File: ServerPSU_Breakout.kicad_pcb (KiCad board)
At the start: 2 copper layers, 91.4 x 69.8 mm, 4 parts

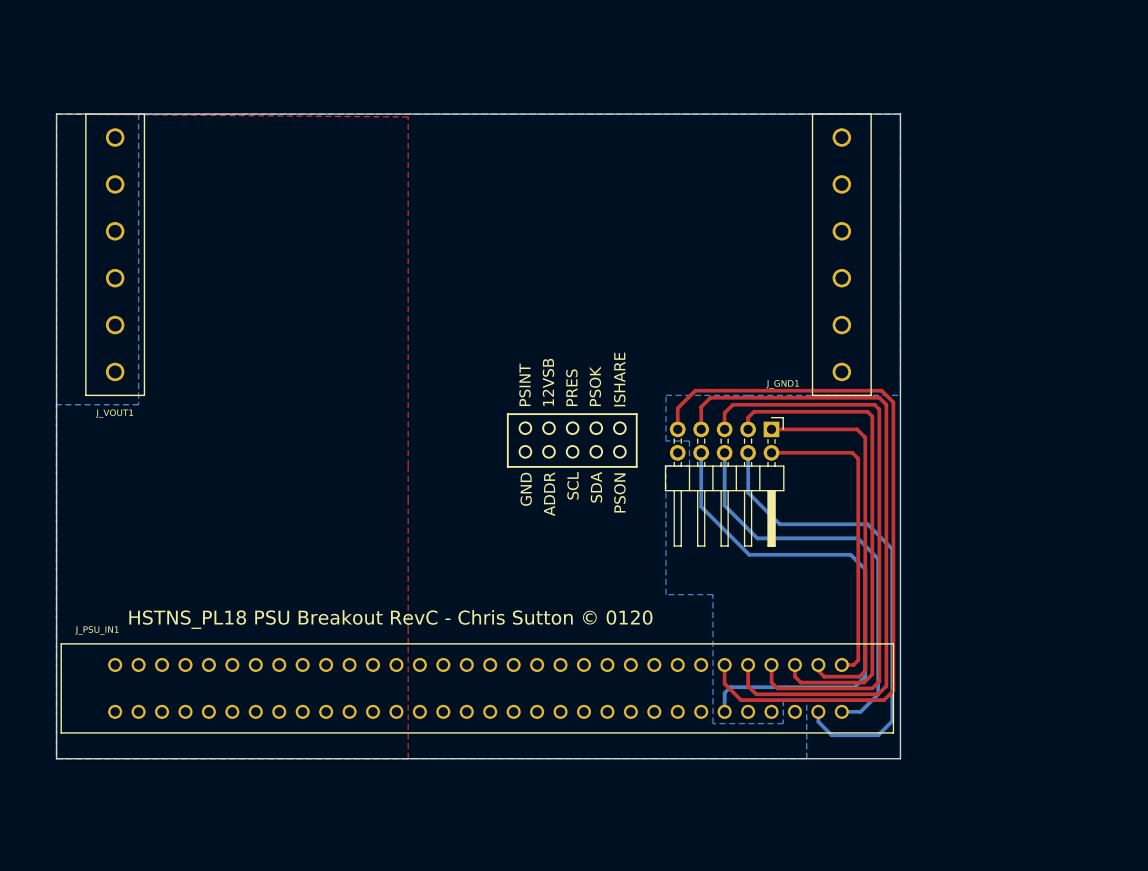
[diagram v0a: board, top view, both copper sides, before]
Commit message: layout draft
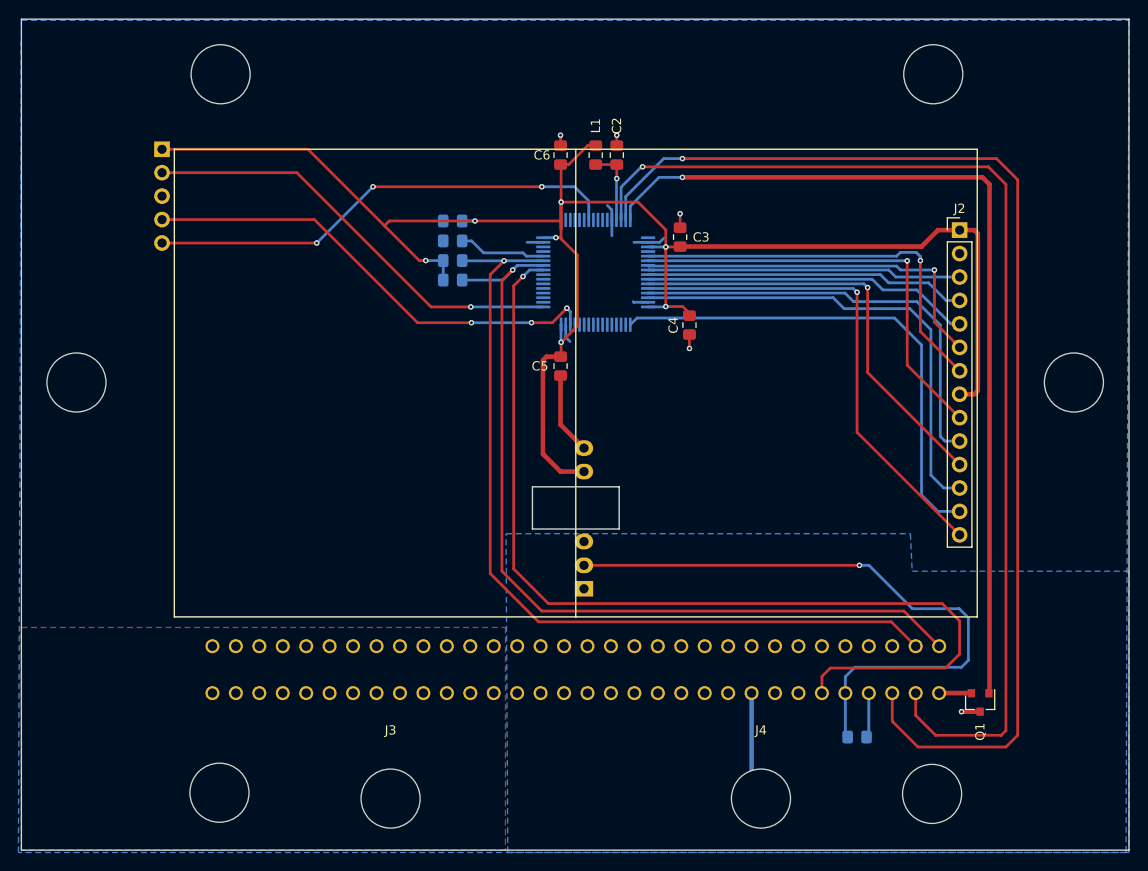
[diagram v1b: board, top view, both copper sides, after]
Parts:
- removed J_DATA1: 2x5_2.54mm, Connector_PinHeader_2.54mm:PinHeader_2x05_P2.54mm_Horizontal
- removed J_GND1, J_VOUT1: 1x6_5.08mm, Samtec HPM-06-02-T-S-RA_1x6:Samtec HPM-06-02-T-S-RA_2x6
- added C1: 100nF, Capacitor_SMD:C_0805_2012Metric_Pad1.15x1.40mm_HandSolder, B.Cu at (148.3, 68.7)
- added C2: 100nF, Capacitor_SMD:C_0805_2012Metric_Pad1.15x1.40mm_HandSolder, F.Cu at (166.1, 61.6)
- added C3: 100nF, Capacitor_SMD:C_0805_2012Metric_Pad1.15x1.40mm_HandSolder, F.Cu at (173.0, 70.5)
- added C4: 100nF, Capacitor_SMD:C_0805_2012Metric_Pad1.15x1.40mm_HandSolder, F.Cu at (174.0, 80.0)
- added C5: 100nF, Capacitor_SMD:C_0805_2012Metric_Pad1.15x1.40mm_HandSolder, F.Cu at (160.0, 84.5)
- added C6: 100nF, Capacitor_SMD:C_0805_2012Metric_Pad1.15x1.40mm_HandSolder, F.Cu at (160.0, 61.6)
- added J1: Conn_01x05, Connector_PinHeader_2.54mm:PinHeader_1x05_P2.54mm_Vertical, B.Cu at (116.8, 61.0)
- added J2: Conn_01x14, Connector_PinHeader_2.54mm:PinHeader_1x14_P2.54mm_Vertical, F.Cu at (203.3, 69.7)
- added J3: Conn_01x01, MountingHole:MountingHole_6.4mm_M6, F.Cu at (141.6, 131.3)
- added J4: Conn_01x01, MountingHole:MountingHole_6.4mm_M6, F.Cu at (181.7, 131.3)
- added L1: BEAD, Inductor_SMD:L_0805_2012Metric_Pad1.15x1.40mm_HandSolder, F.Cu at (163.8, 61.6)
- added Q1: DMG2302U, Package_TO_SOT_SMD:SOT-23, F.Cu at (205.5, 120.9)
- added R1: 10K, Resistor_SMD:R_0805_2012Metric_Pad1.15x1.40mm_HandSolder, B.Cu at (148.3, 75.1)
- added R2: 10K, Resistor_SMD:R_0805_2012Metric_Pad1.15x1.40mm_HandSolder, B.Cu at (148.3, 73.0)
- added R3: 22K, Resistor_SMD:R_0805_2012Metric_Pad1.15x1.40mm_HandSolder, B.Cu at (192.2, 124.7)
- added R4: 10K, Resistor_SMD:R_0805_2012Metric_Pad1.15x1.40mm_HandSolder, B.Cu at (148.3, 70.9)
- added REF**: MountingHole_6.4mm_M6, MountingHole:MountingHole_6.4mm_M6, F.Cu at (215.6, 86.2)
- added REF**: MountingHole_6.4mm_M6, MountingHole:MountingHole_6.4mm_M6, F.Cu at (107.6, 86.2)
- added REF**: MountingHole_6.4mm_M6, MountingHole:MountingHole_6.4mm_M6, F.Cu at (200.3, 130.8)
- added REF**: MountingHole_6.4mm_M6, MountingHole:MountingHole_6.4mm_M6, F.Cu at (123.1, 130.7)
- added REF**: MountingHole_6.4mm_M6, MountingHole:MountingHole_6.4mm_M6, F.Cu at (200.4, 52.8)
- added REF**: MountingHole_6.4mm_M6, MountingHole:MountingHole_6.4mm_M6, F.Cu at (123.2, 52.8)
- added U1: NCS1S1203SC, Converter_DCDC:Converter_DCDC_Murata_NCS1SxxxxSC_THT, B.Cu at (162.6, 108.6)
- added U2: STM32F072RBTx, Package_QFP:LQFP-64_10x10mm_P0.5mm, B.Cu at (163.8, 74.3)
- J_PSU_IN1: moved to B.Cu
- moved J_PSU_IN1 10.7 mm to (161.7, 117.3), turned to 270 degrees
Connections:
- net /12V renamed /OutputConnectors/PSU_VBUS
- net /GND renamed GNDS
- J_PSU_IN1 pad 27: /ADDR -> /PSUConnector/PSU_ADDR2
- J_PSU_IN1 pad 28: Net-(J_PSU_IN1-Pad28) -> /PSUConnector/PSU_ADDR1
- J_PSU_IN1 pad 29: Net-(J_PSU_IN1-Pad29) -> /PSUConnector/PSU_ADDR0
- J_PSU_IN1 pad 31: /SDA -> /PSUConnector/PSU_SDA
- J_PSU_IN1 pad 32: /SCL -> /PSUConnector/PSU_SCL
- J_PSU_IN1 pad 33: /PSON -> /HighVoltageControl/PSU_ON
- J_PSU_IN1 pad 34: /ISHARE -> /MCU/MCU_IMON
- J_PSU_IN1 pad 35: /PSOK -> /MCU/MCU_PSOK
- J_PSU_IN1 pad 36: /PRESENT -> /HighVoltageControl/PSU_PRES
- J_PSU_IN1 pad 37: /12VSB -> /HighVoltageControl/PSU_12VSB
- J_PSU_IN1 pad 38: /PSINTERRUPT -> /PSUConnector/PSU_INT
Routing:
- net /HighVoltageControl/MCU_3V3: track 0.00 -> 193.4 mm, vias 0 -> 7
- net /MCU/MCU_PSOK: track 0.00 -> 126.2 mm, vias 0 -> 1
- net /MCU/MCU_IMON: track 0.00 -> 119.4 mm, vias 0 -> 1
- net /PSUConnector/PSU_INT: track 0.00 -> 106.6 mm, vias 0 -> 1
- net /HighVoltageControl/MCU_SW: track 0.00 -> 97.2 mm, vias 0 -> 1
- net /PSUConnector/PSU_SCL: track 0.00 -> 93.3 mm, vias 0 -> 1
- net /PSUConnector/PSU_SDA: track 0.00 -> 92.7 mm, vias 0 -> 1
- net /PSINTERRUPT: track 79.7 -> 0.00 mm
- net /12VSB: track 71.7 -> 0.00 mm
- net /HighVoltageControl/PSU_12VSB: track 0.00 -> 69.4 mm, vias 0 -> 1
- net /PRESENT: track 62.8 -> 0.00 mm
- net /ADDR: track 56.1 -> 0.00 mm
- net /MCU/T_OUT: track 0.00 -> 54.2 mm
- net /MCU/T_IRQ: track 0.00 -> 53.7 mm, vias 0 -> 1
- net /PSOK: track 53.4 -> 0.00 mm
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- added copper zone on B.Cu, net /HighVoltageControl/MCU_GND
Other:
- board size 91.4 x 69.8 mm -> 120 x 90 mm
- net class Default: clearance 0.2 -> 0.127; trace_width 0.25 -> 0.127; via_dia 0.8 -> 0.6; via_drill 0.4 -> 0.3
- rule trace_clearance: 0.2 -> 0.127
- rule trace_min: 0.2 -> 0.127
- rule via_min_size: 0.4 -> 0.6
- board text removed: "12VSB"
- board text removed: "ADDR"
- board text removed: "GND"
- board text removed: "HSTNS_PL18 PSU Breakout RevC - Chris Sutton © 0120"
- board text removed: "ISHARE"
- board text removed: "PRES"
- board text removed: "PSINT"
- board text removed: "PSOK"
- board text removed: "PSON"
- board text removed: "SCL"
- board text removed: "SDA"
